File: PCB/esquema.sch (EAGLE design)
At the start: 11 parts, among them U1 ATMEGA328P_TQFP

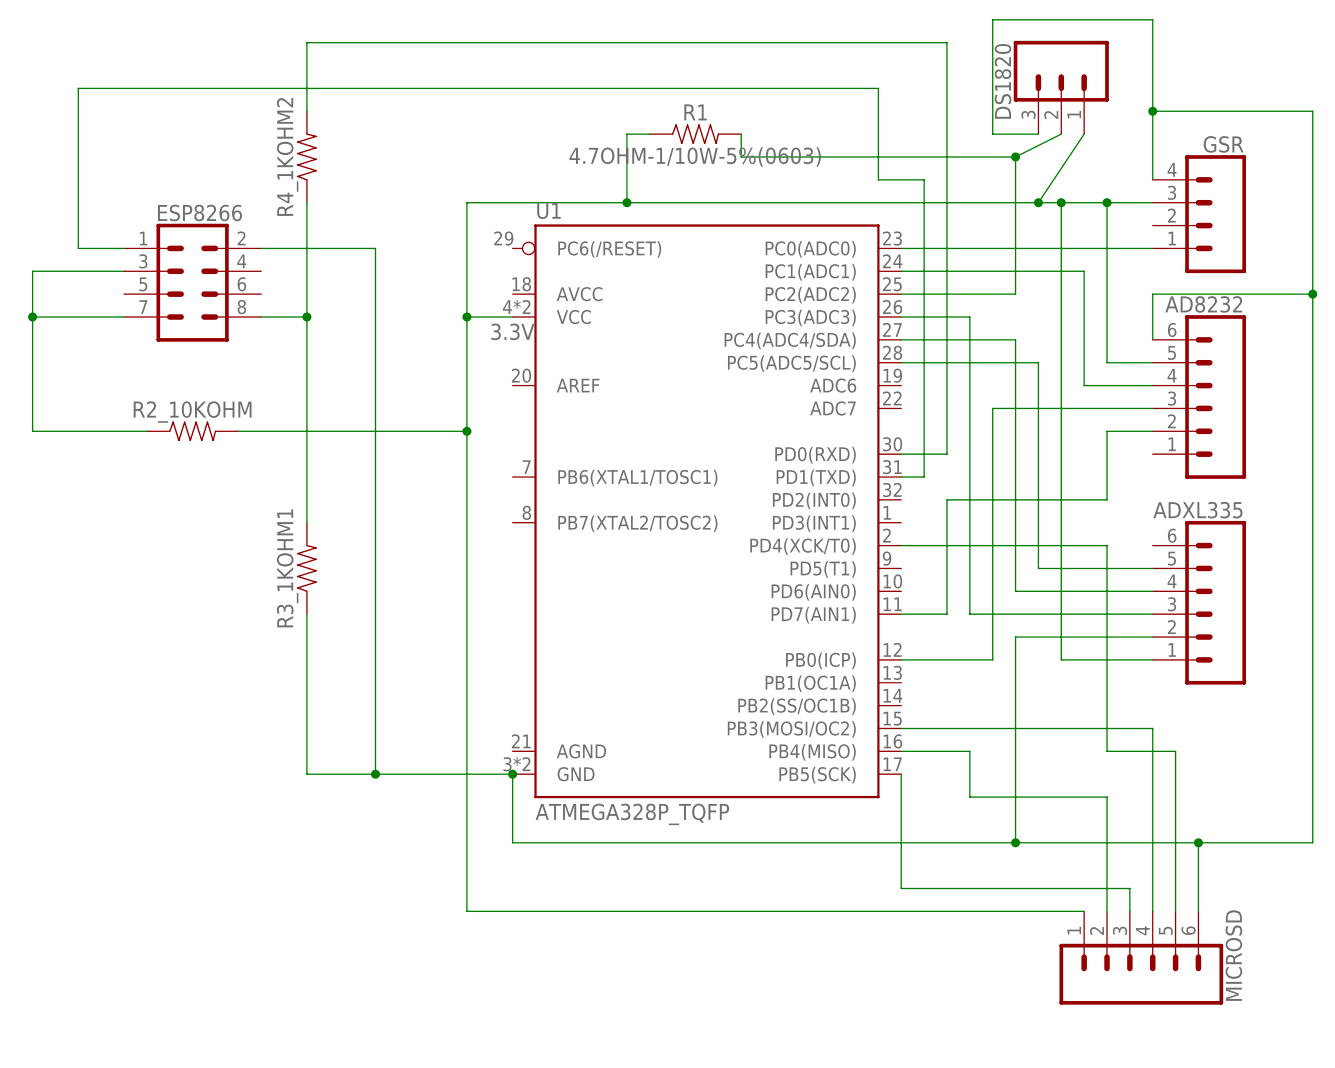
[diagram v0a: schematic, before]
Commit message: Fin PCB
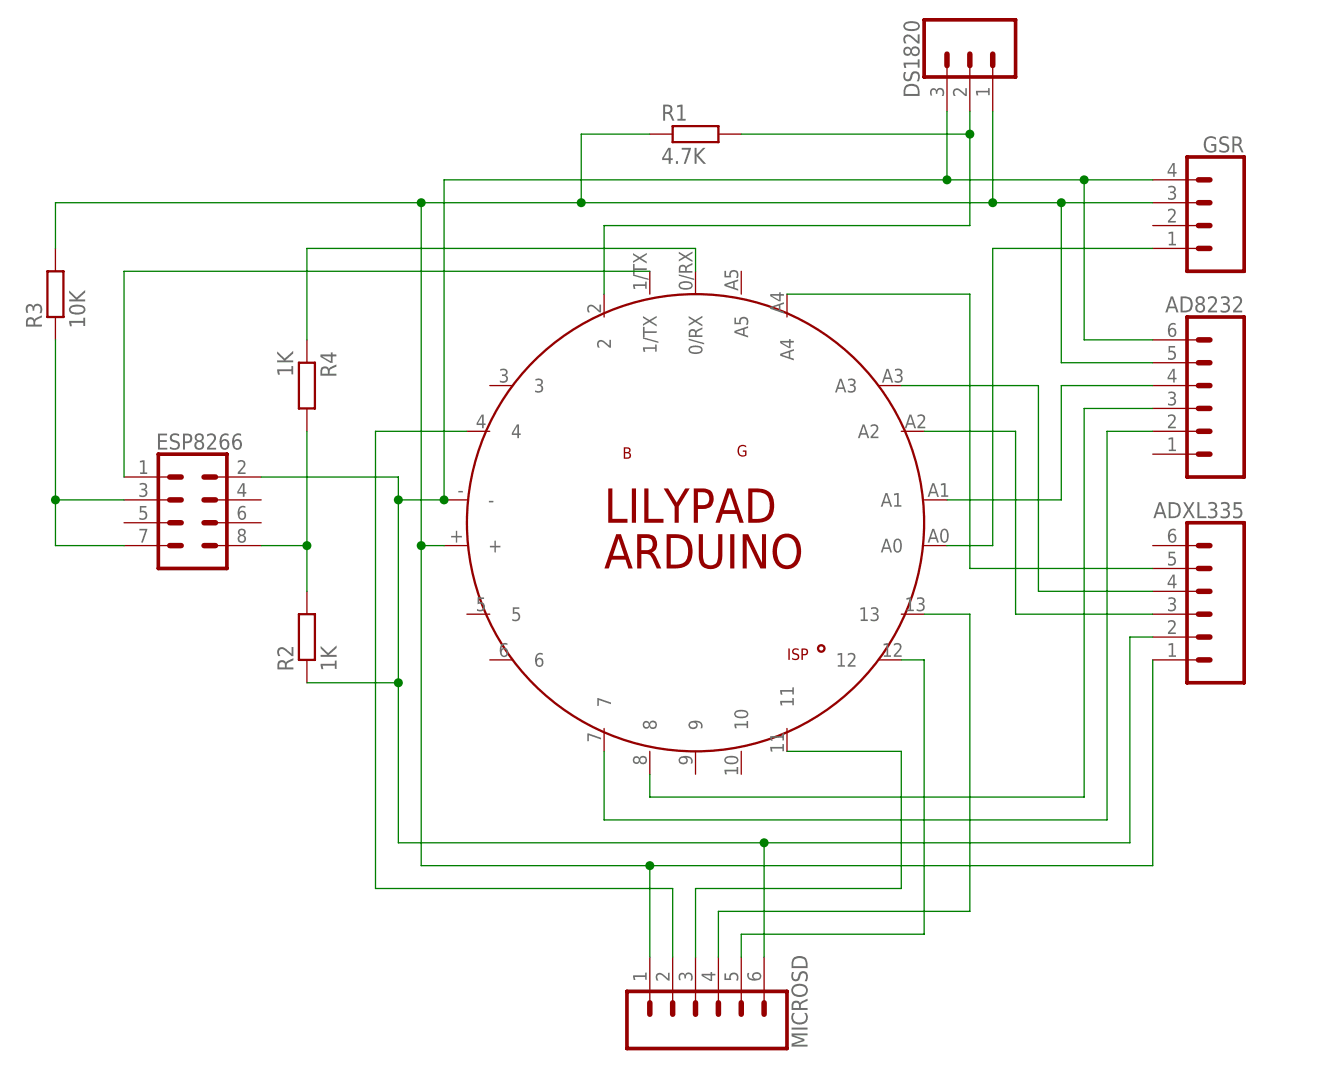
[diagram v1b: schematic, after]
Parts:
- removed R2_10KOHM, R3_1KOHM1, R4_1KOHM2: 2.2MOHM-1/10W-5%(0603), SparkFun-Retired:2.2MOHM-1/10W-5%(0603)
- removed U1: ATMEGA328P_TQFP, SparkFun-IC-Microcontroller:ATMEGA328P_TQFP
- added PCB1: ARDUINO_LILYPAD, E14_Arduino_revB:ARDUINO_LILYPAD
- added R2, R4: 1K, rcl:R-EU_0309/12
- added R3: 10K, rcl:R-EU_0309/12
- R1: value 4.7OHM-1/10W-5%(0603) -> 4.7K; device SparkFun-Retired:4.7OHM-1/10W-5%(0603) -> rcl:R-EU_0309/12
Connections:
- removed net 3.3V: AD8232.5, ADXL335.1, DS1820.1, GSR.3, MICROSD.1, R1.1, R2_10KOHM.2, U1.VCC
- new net N$18: MICROSD.5, PCB1.12
- net N$1: now also MICROSD.3, PCB1.11; no longer AD8232.6, ADXL335.2, DS1820.3, ESP8266.2, GSR.4, MICROSD.6, R3_1KOHM1.1, U1.GND
- net N$10: now also R3.1; no longer R2_10KOHM.1
- net N$11: now also ADXL335.5, PCB1.A4; no longer ESP8266.1, U1.PD1(TXD)
- net N$12: now also ESP8266.1, PCB1.1/TX; no longer ESP8266.8, R3_1KOHM1.2, R4_1KOHM2.1
- net N$13: now also ESP8266.8, R2.2, R4.2; no longer AD8232.2, U1.PD7(AIN1)
- net N$14: now also PCB1.0/RX, R4.1; no longer R4_1KOHM2.2, U1.PD0(RXD)
- net N$15: now also AD8232.5, ADXL335.1, DS1820.1, GSR.3, MICROSD.1, PCB1.+, R1.1, R3.2; no longer MICROSD.2, U1.PB4(MISO)
- net N$16: now also AD8232.6, ADXL335.2, DS1820.3, ESP8266.2, GSR.4, MICROSD.6, PCB1.-, R2.1; no longer MICROSD.3, U1.PB5(SCK)
- net N$17: now also PCB1.13; no longer U1.PB3(MOSI/OC2)
- net N$2: now also MICROSD.2, PCB1.4; no longer GSR.1, U1.PC0(ADC0)
- net N$3: now also GSR.1, PCB1.A0; no longer AD8232.4, U1.PC1(ADC1)
- net N$4: now also AD8232.4, PCB1.A1; no longer AD8232.3, U1.PB0(ICP)
- net N$5: now also AD8232.3, PCB1.8; no longer MICROSD.5, U1.PD4(XCK/T0)
- net N$6: now also AD8232.2, PCB1.7; no longer ADXL335.3, U1.PC3(ADC3)
- net N$7: now also PCB1.2; no longer U1.PC2(ADC2)
- net N$8: now also ADXL335.3, PCB1.A2; no longer ADXL335.4, U1.PC4(ADC4/SDA)
- net N$9: now also ADXL335.4, PCB1.A3; no longer ADXL335.5, U1.PC5(ADC5/SCL)
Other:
- moved on the sheet: DS1820, ESP8266, MICROSD
